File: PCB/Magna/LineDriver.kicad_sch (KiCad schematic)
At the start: 36 parts, among them J1301 Conn_Coaxial, J1302 Conn_Coaxial, U1301 NE5532, U1302 NE5532, U1303 NE5532

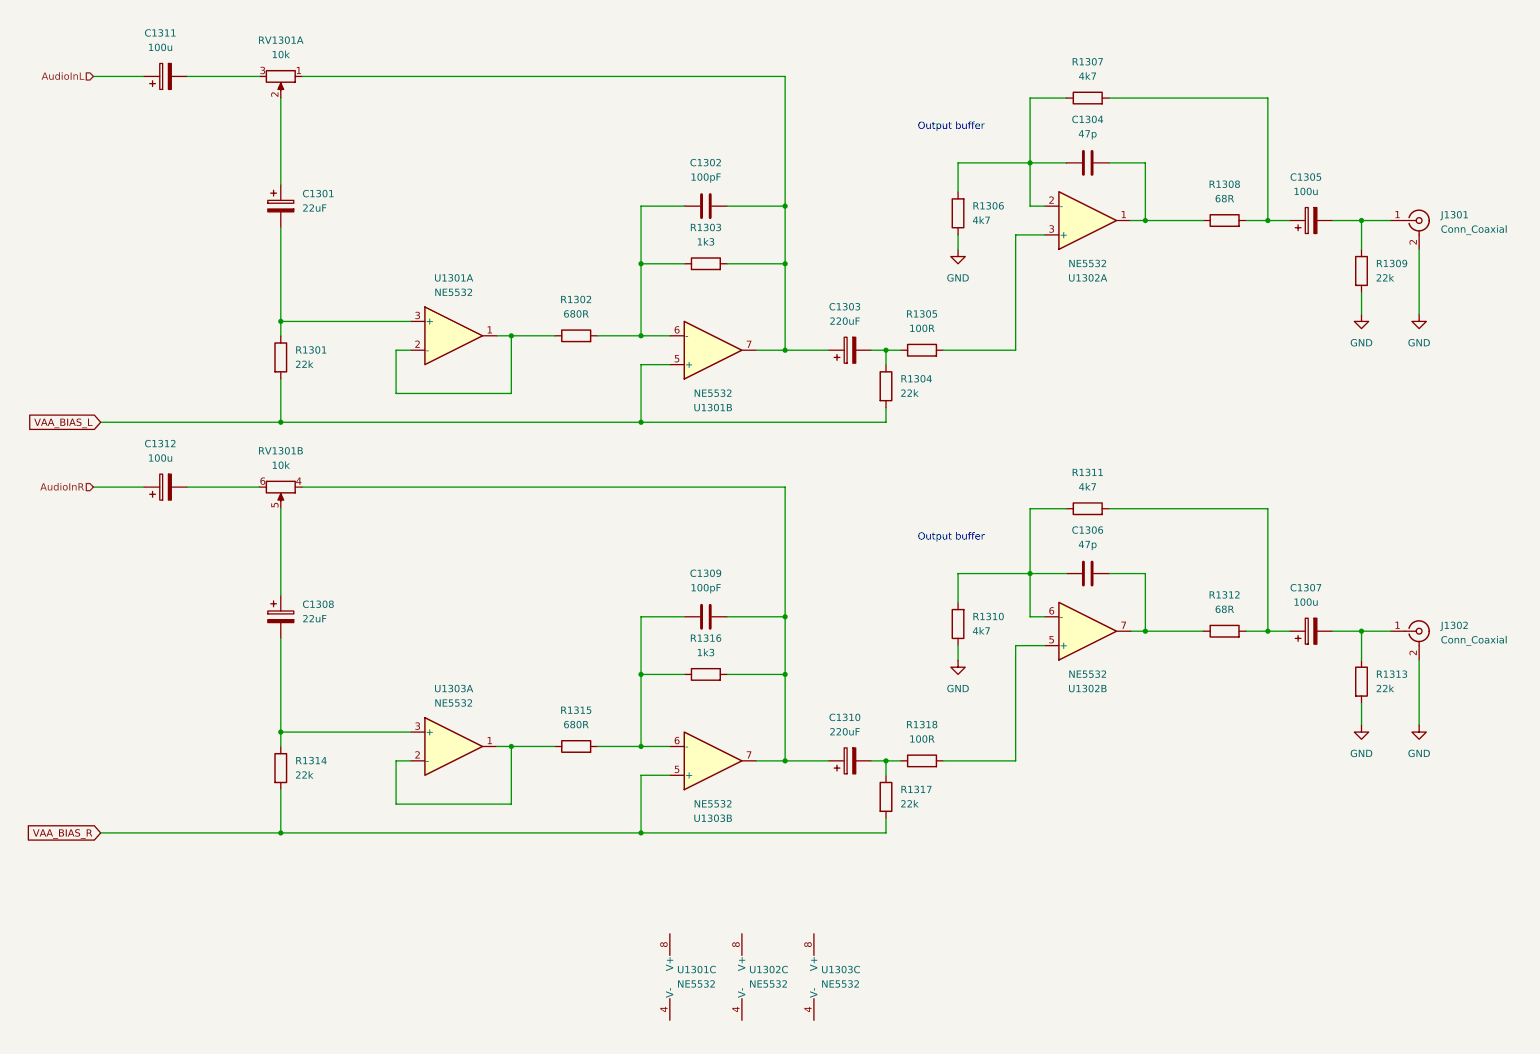
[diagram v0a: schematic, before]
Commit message: Add final touched to all schematics
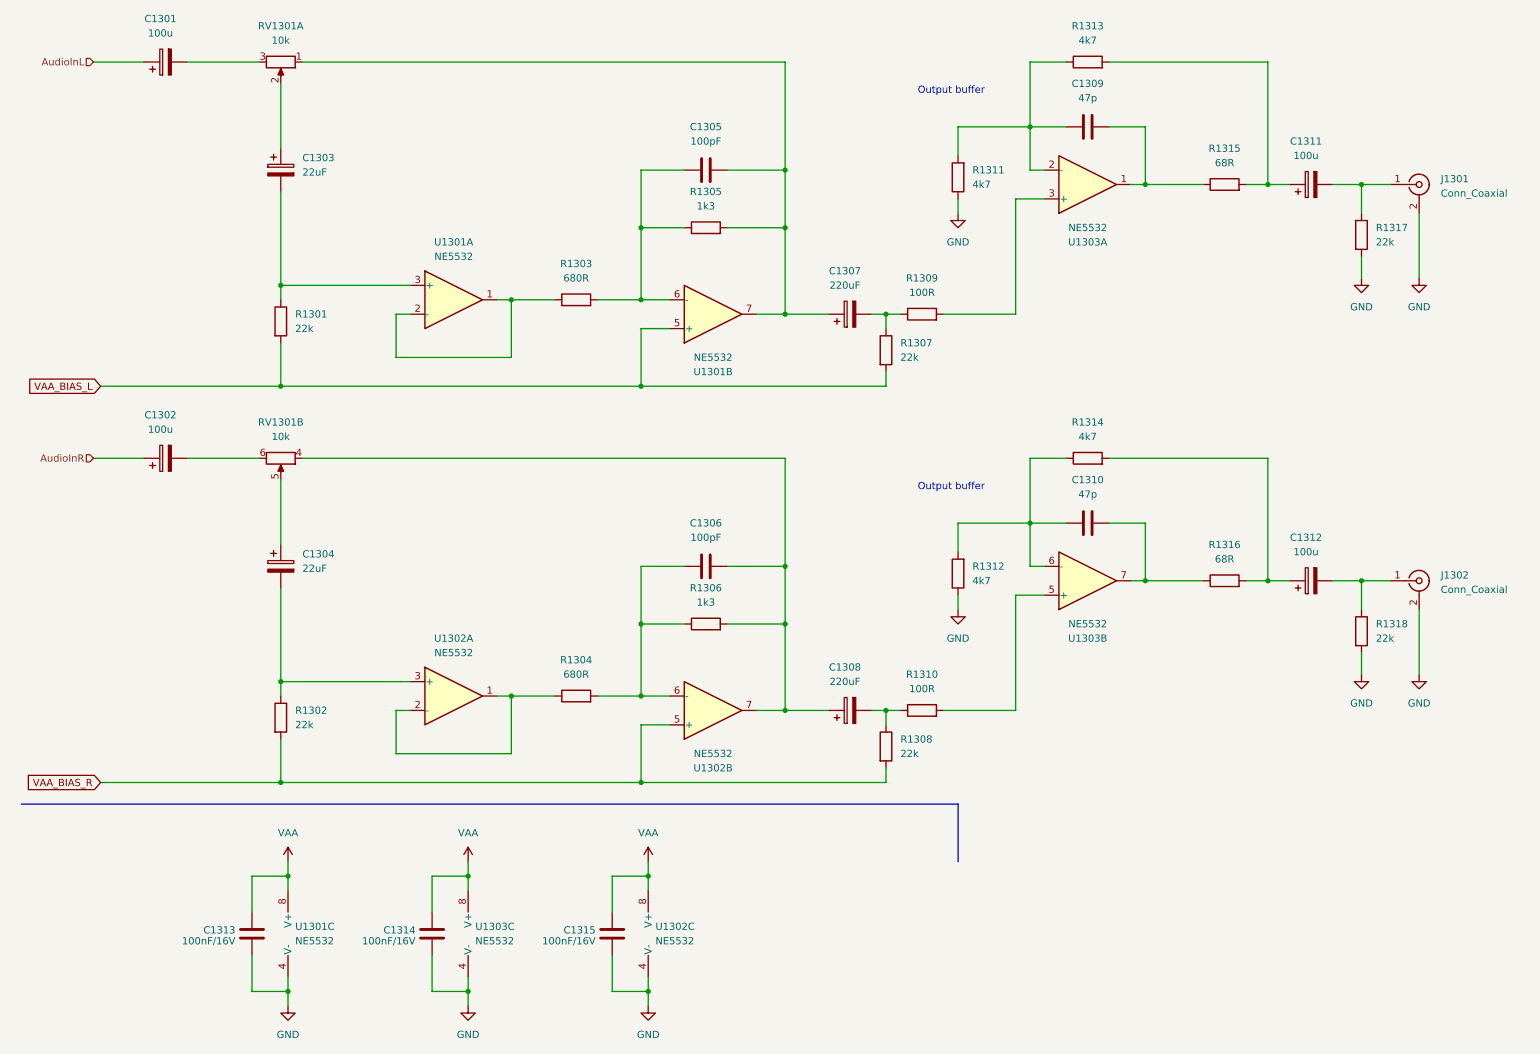
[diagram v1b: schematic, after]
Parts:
- added C1313, C1314, C1315: 100nF/16V, Capacitor_SMD:C_0402_1005Metric, symbol Device:C
- renumbered C1311 to C1301, C1312 to C1302, C1301 to C1303, C1308 to C1304, C1302 to C1305, C1309 to C1306, C1303 to C1307, C1310 to C1308, C1304 to C1309, C1306 to C1310, C1305 to C1311, C1307 to C1312, R1314 to R1302, R1302 to R1303, R1315 to R1304, R1303 to R1305, R1316 to R1306, R1304 to R1307, R1317 to R1308, R1305 to R1309, R1318 to R1310, R1306 to R1311, R1310 to R1312, R1307 to R1313, R1311 to R1314, R1308 to R1315, R1312 to R1316, R1309 to R1317, R1313 to R1318, U1303 to U1302, U1302 to U1303
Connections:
- net GND: now also U1301.4 (V-), U1302.4 (V-), U1303.4 (V-), C1313.2, C1314.2, C1315.2
- net VAA: now reaches U1301.8 (V+)
- net VAA: now also U1302.8 (V+), U1303.8 (V+), C1313.1, C1314.1, C1315.1
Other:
- moved on the sheet: C1301, C1302, C1303, C1304, C1305, C1306, C1307, C1308, C1309, C1310, C1311, C1312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
